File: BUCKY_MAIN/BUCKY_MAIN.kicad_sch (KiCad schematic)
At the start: 17 parts, among them J4 Conn_01x10, U1 IFX9201SG_BO, U2 IFX9201SG_BO, U3 IFX9201SG_BO, U9 PCA9548ADB

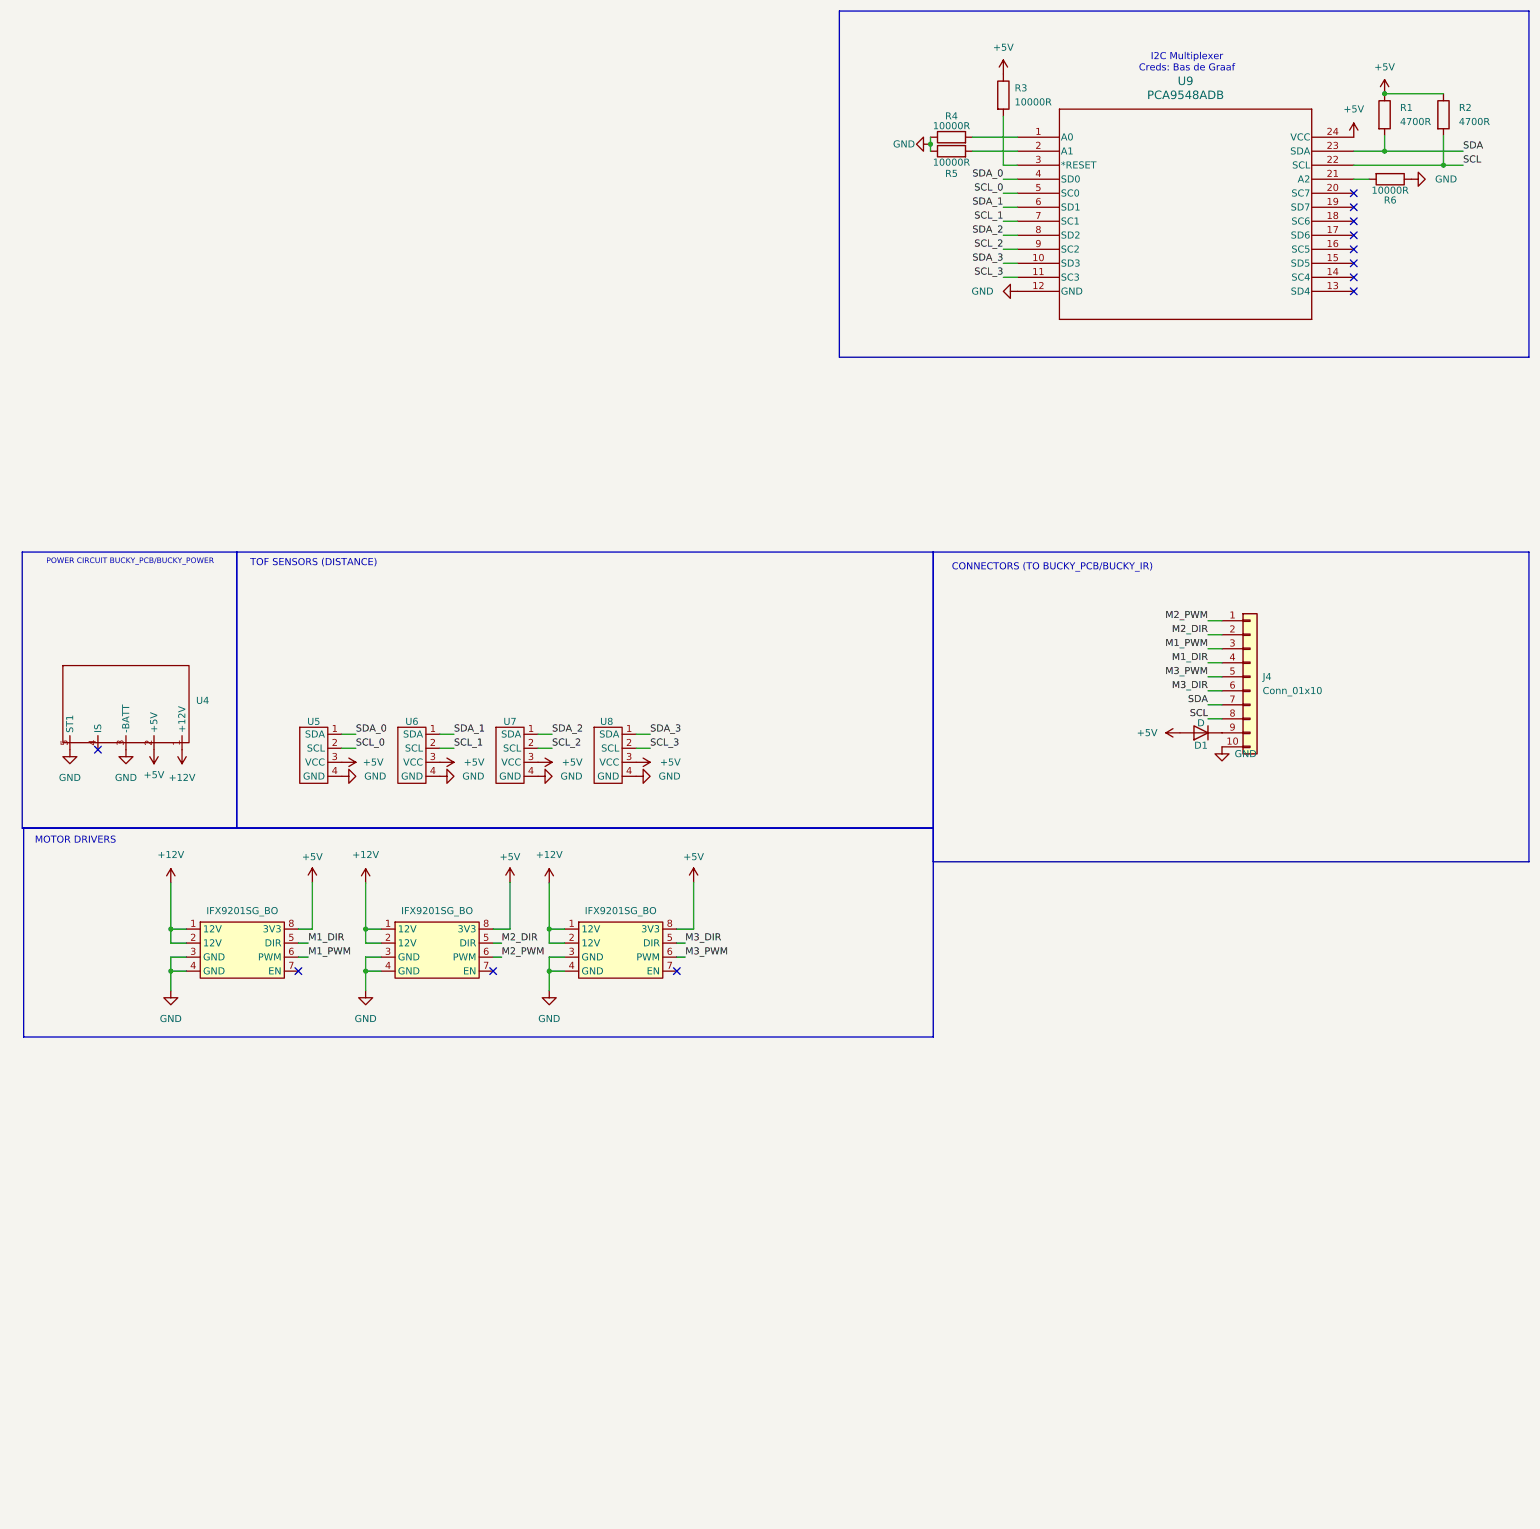
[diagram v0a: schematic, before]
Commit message: chore: finish main board
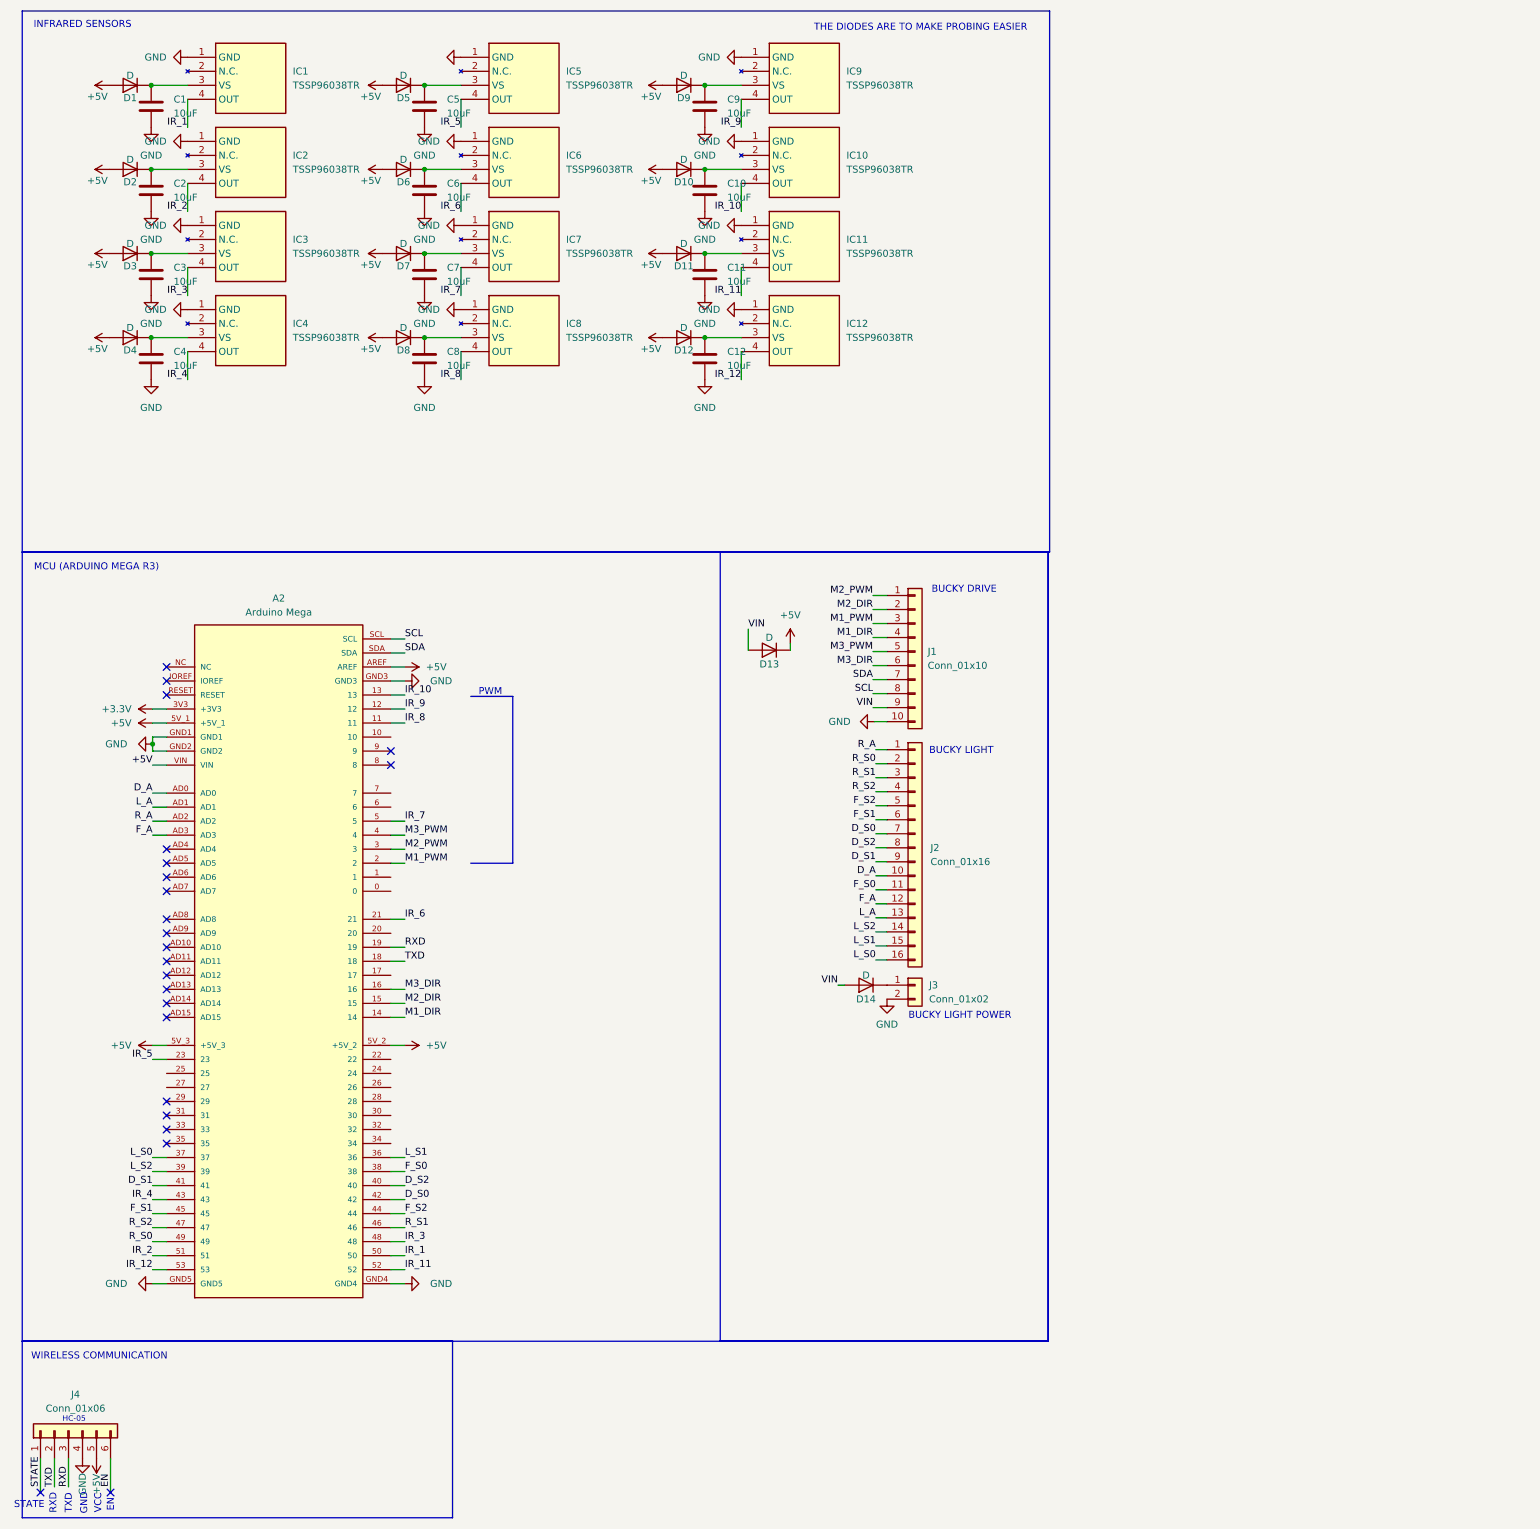
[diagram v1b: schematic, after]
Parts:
- removed J4: Conn_01x10, BUCKY_MAIN:CONN10_S10B-PH_JST, symbol Connector_Generic:Conn_01x10
- removed R1, R2: 4700R, Resistor_SMD:R_0402_1005Metric, symbol Device:R
- removed R3, R4, R5, R6: 10000R, Resistor_SMD:R_0402_1005Metric, symbol Device:R
- removed U1, U2, U3: IFX9201SG_BO, BUCKY_MAIN:IFX9201SG_BO, symbol BUCKY_MAIN:IFX9201SG_BO
- removed U4: ~, BUCKY_MAIN:BUCKY_POWER, symbol BUCKY_MAIN:BUCKY_POWER
- removed U5, U6, U7, U8: ~, BUCKY_MAIN:BUCKY_TOF, symbol BUCKY_MAIN:BUCKY_TOF
- removed U9: PCA9548ADB, DB24, symbol BUCKY_MULTIPLEXER:PCA9548ADB
- added A2: Arduino Mega, BUCKY_MAIN:ARDUINO_MEGA, symbol ARDUINO_MEGA:A000067
- added C1, C10, C11, C12, C2, C3, C4, C5, C6, C7, C8, C9: 10uF, Capacitor_SMD:C_0603_1608Metric, symbol Device:C
- added D10, D11, D12, D13, D14, D2, D3, D4, D5, D6, D7, D8, D9: D, Diode_SMD:D_0603_1608Metric, symbol Device:D
- added IC1, IC10, IC11, IC12, IC2, IC3, IC4, IC5, IC6, IC7, IC8, IC9: TSSP96038TR, BUCKY_MAIN:TSSP96038, symbol BUCKY_MAIN:TSSP96038TR
- added J1: Conn_01x10, BUCKY_MAIN:CONN10_S10B-PH_JST, symbol Connector_Generic:Conn_01x10
- added J2: Conn_01x16, BUCKY_MAIN:CONN_B16B-PH-SM4-TB_JST, symbol Connector_Generic:Conn_01x16
- added J3: Conn_01x02, BUCKY_MAIN:CONN_S2B-PH-K-S_JST, symbol Connector_Generic:Conn_01x02
- added J4: Conn_01x06, Connector_PinHeader_2.54mm:PinHeader_1x06_P2.54mm_Horizontal, symbol Connector_Generic:Conn_01x06
- D1: footprint (none) -> Diode_SMD:D_0603_1608Metric
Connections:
- net +5V: now also A2.5V_1 (+5V_1), A2.5V_2 (+5V_2), A2.5V_3 (+5V_3), A2.AREF, A2.VIN, D10.2 (A), D11.2 (A), D12.2 (A), D13.1 (K), D2.2 (A), D3.2 (A), D4.2 (A), D5.2 (A), D6.2 (A), D7.2 (A), D8.2 (A), D9.2 (A), J4.5 (Pin_5)
- net GND: now also A2.GND1, A2.GND2, A2.GND3, A2.GND4, A2.GND5, C1.1, C10.1, C11.1, C12.1, C2.1, C3.1, C4.1, C5.1, C6.1, C7.1, C8.1, C9.1, IC1.1 (GND), IC10.1 (GND), IC11.1 (GND), IC12.1 (GND), IC2.1 (GND), IC3.1 (GND), IC4.1 (GND), IC5.1 (GND), IC6.1 (GND), IC7.1 (GND), IC8.1 (GND), IC9.1 (GND), J1.10 (Pin_10), J3.2 (Pin_2), J4.4 (Pin_4)
- net M1_DIR: now also A2.14, J1.4 (Pin_4)
- net M1_PWM: now also A2.2, J1.3 (Pin_3)
- net M2_DIR: now also A2.15, J1.2 (Pin_2)
- net M2_PWM: now also A2.3, J1.1 (Pin_1)
- net M3_DIR: now also A2.16, J1.6 (Pin_6)
- net M3_PWM: now also A2.4, J1.5 (Pin_5)
- net SCL: now also A2.SCL, J1.8 (Pin_8)
- net SDA: now also A2.SDA, J1.7 (Pin_7)
- net at D1.1 (K): now also C1.2, IC1.3 (VS)
- new net: C3.2, D3.1 (K), IC3.3 (VS)
- new net: C8.2, D8.1 (K), IC8.3 (VS)
- new net: C4.2, D4.1 (K), IC4.3 (VS)
- new net: C10.2, D10.1 (K), IC10.3 (VS)
- new net: C2.2, D2.1 (K), IC2.3 (VS)
- new net: C11.2, D11.1 (K), IC11.3 (VS)
- new net: C6.2, D6.1 (K), IC6.3 (VS)
- new net: C9.2, D9.1 (K), IC9.3 (VS)
- new net: C5.2, D5.1 (K), IC5.3 (VS)
- new net: C7.2, D7.1 (K), IC7.3 (VS)
- new net: C12.2, D12.1 (K), IC12.3 (VS)
- new net: D14.1 (K), J3.1 (Pin_1)
- new net +3.3V: A2.3V3 (+3V3)
- new net D_A: A2.AD0, J2.10 (Pin_10)
- new net D_S0: A2.42, J2.7 (Pin_7)
- new net D_S1: A2.41, J2.9 (Pin_9)
- new net D_S2: A2.40, J2.8 (Pin_8)
- new net EN: J4.6 (Pin_6)
- new net F_A: A2.AD3, J2.12 (Pin_12)
- new net F_S0: A2.38, J2.11 (Pin_11)
- new net F_S1: A2.45, J2.6 (Pin_6)
- new net F_S2: A2.44, J2.5 (Pin_5)
- new net IR_1: A2.50, IC1.4 (OUT)
- new net IR_10: A2.13, IC10.4 (OUT)
- new net IR_11: A2.52, IC11.4 (OUT)
- new net IR_12: A2.53, IC12.4 (OUT)
- new net IR_2: A2.51, IC2.4 (OUT)
- new net IR_3: A2.48, IC3.4 (OUT)
- new net IR_4: A2.43, IC4.4 (OUT)
- new net IR_5: A2.23, IC5.4 (OUT)
- new net IR_6: A2.21, IC6.4 (OUT)
- new net IR_7: A2.5, IC7.4 (OUT)
- new net IR_8: A2.11, IC8.4 (OUT)
- new net IR_9: A2.12, IC9.4 (OUT)
- new net L_A: A2.AD1, J2.13 (Pin_13)
- new net L_S0: A2.37, J2.16 (Pin_16)
- new net L_S1: A2.36, J2.15 (Pin_15)
- new net L_S2: A2.39, J2.14 (Pin_14)
- new net RXD: A2.19, J4.3 (Pin_3)
- new net R_A: A2.AD2, J2.1 (Pin_1)
- new net R_S0: A2.49, J2.2 (Pin_2)
- new net R_S1: A2.46, J2.3 (Pin_3)
- new net R_S2: A2.47, J2.4 (Pin_4)
- new net STATE: J4.1 (Pin_1)
- new net TXD: A2.18, J4.2 (Pin_2)
- new net VIN: D13.2 (A), D14.2 (A), J1.9 (Pin_9)
- no-connect marks 12 -> 23
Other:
- note added: "BUCKY DRIVE"
- note added: "BUCKY LIGHT"
- note added: "BUCKY LIGHT POWER"
- note added: "EN"
- note added: "GND"
- note added: "HC-05"
- note added: "INFRARED SENSORS"
- note added: "MCU (ARDUINO MEGA R3)"
- note added: "PWM"
- note added: "RXD"
- note added: "STATE"
- note added: "THE DIODES ARE TO MAKE PROBING EASIER"
- note added: "TXD"
- note added: "VCC"
- note added: "WIRELESS COMMUNICATION"
- note removed: "CONNECTORS (TO BUCKY_PCB/BUCKY_IR)"
- note removed: "I2C Multiplexer Creds: Bas de Graaf"
- note removed: "MOTOR DRIVERS"
- note removed: "POWER CIRCUIT BUCKY_PCB/BUCKY_POWER"
- note removed: "TOF SENSORS (DISTANCE)"
- title: MAIN BOARD -> BUCKY MAIN
